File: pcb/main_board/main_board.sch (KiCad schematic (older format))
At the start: 32 parts, among them J1 Sensors_Conn, J2 Power_Conn, J3 I2C_Conn, J4 Garage_Conn, J5 Debug_Sensors_Conn, J6 Debug_I2C_Conn, U1 ESP-01, U2 HC_05, U3 AT24CS64-SSHM, U4 AMS1117-3.3, U5 Black_Pill

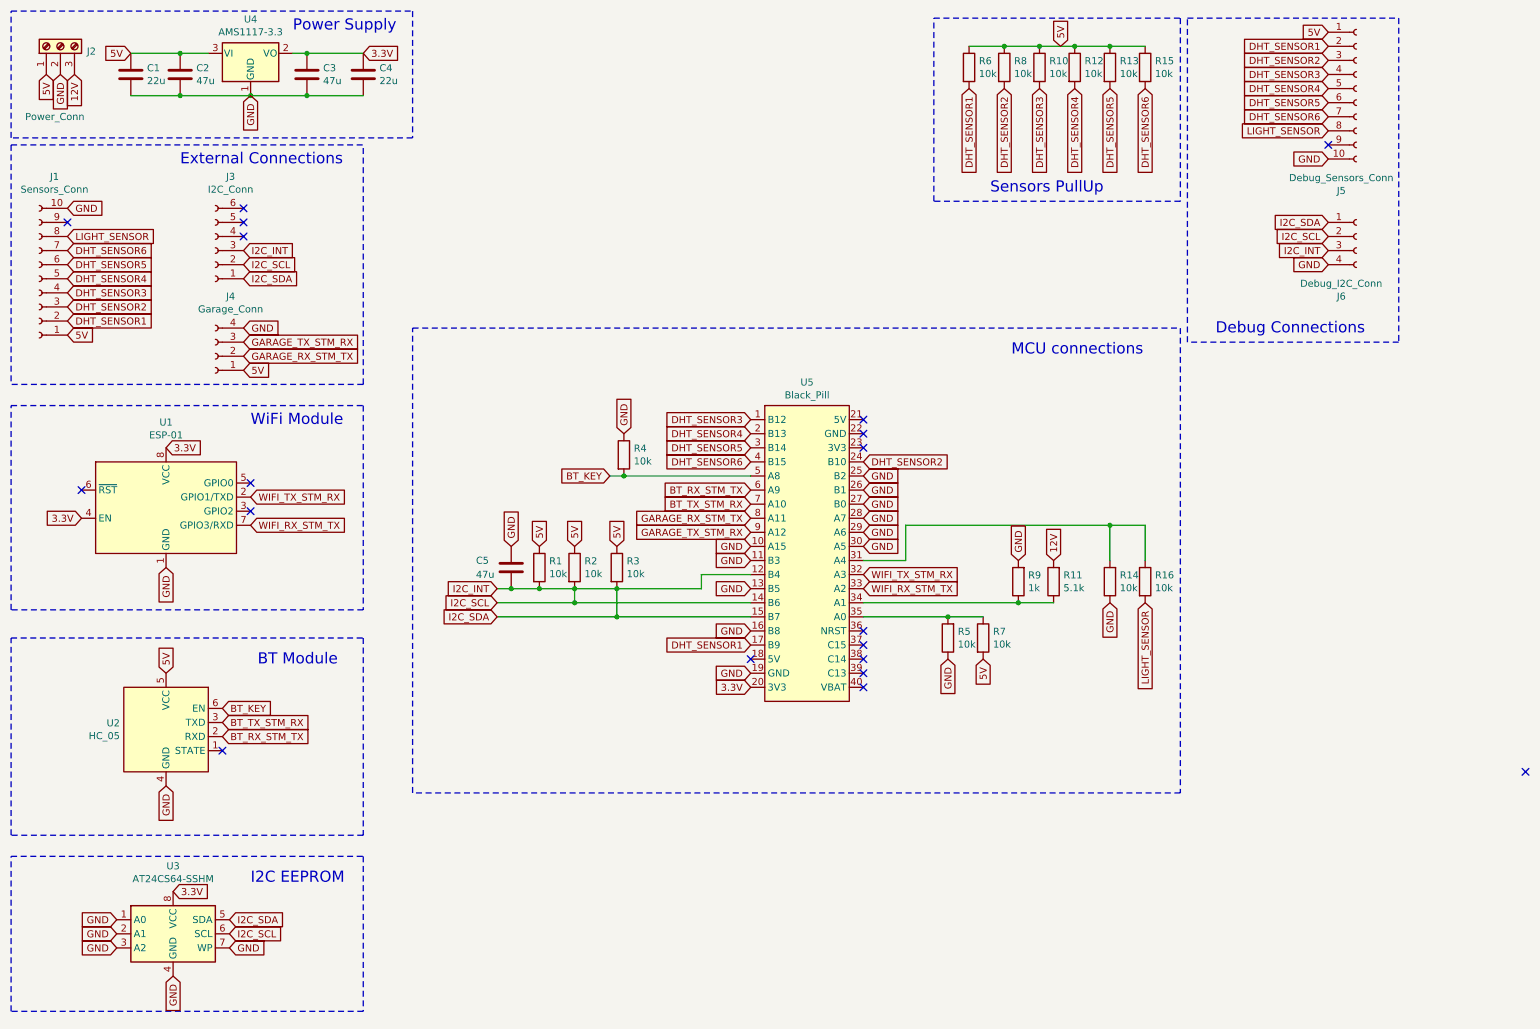
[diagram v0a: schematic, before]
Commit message: PCB layout added
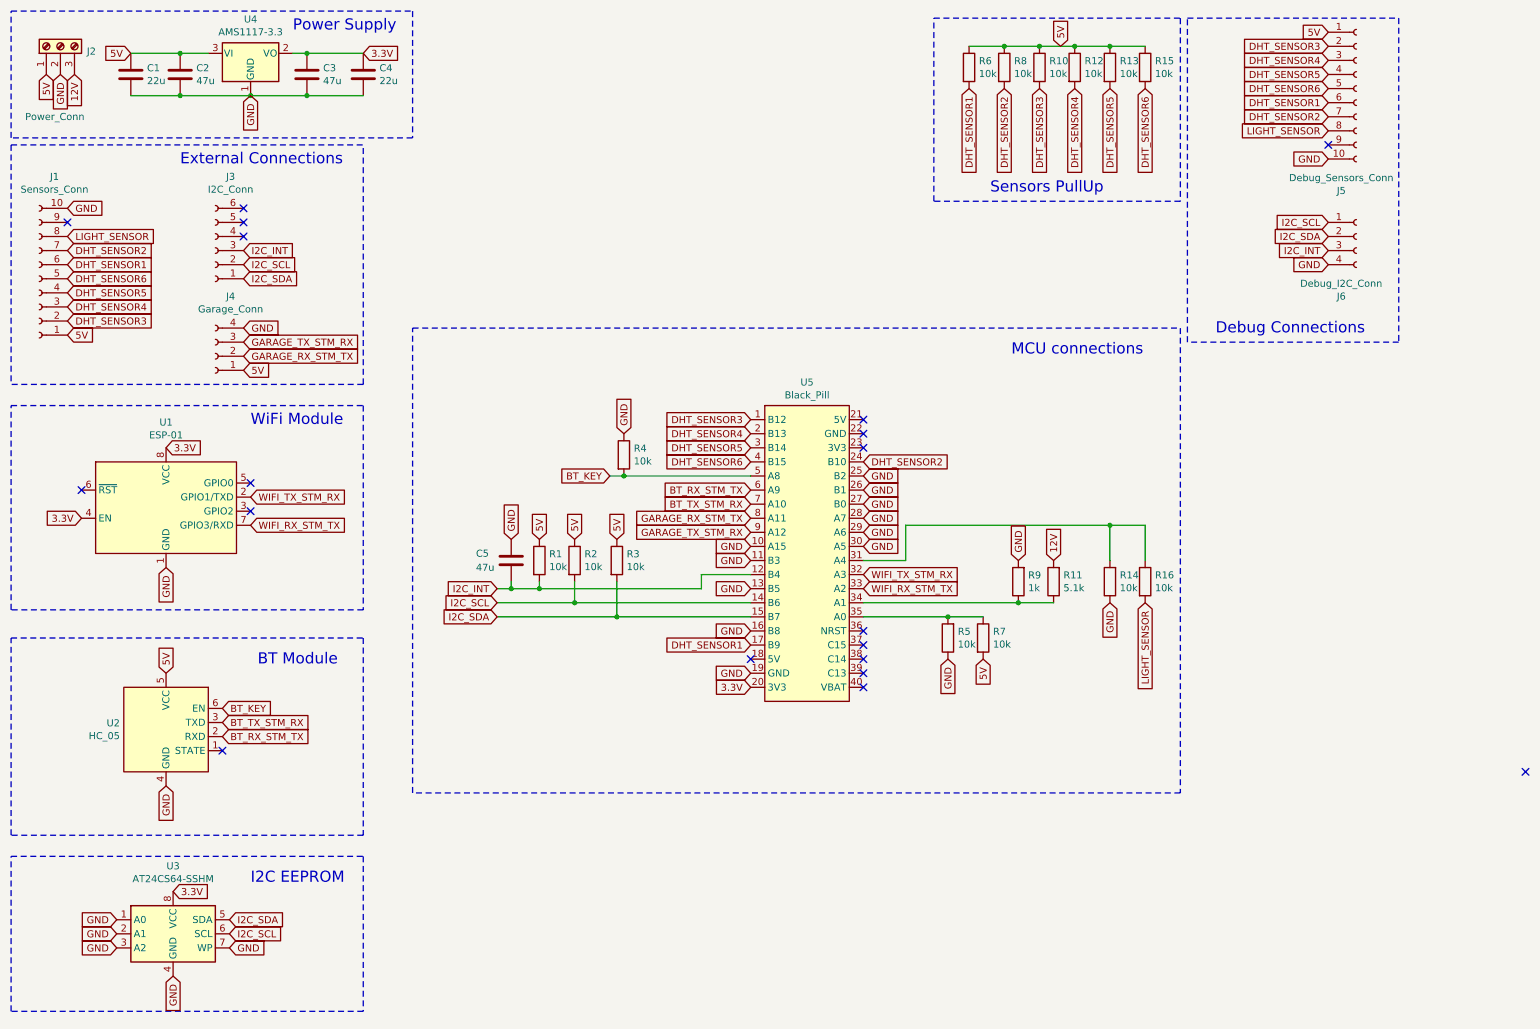
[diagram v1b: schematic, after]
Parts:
- U1: footprint Connector_PinHeader_2.54mm:PinHeader_2x04_P2.54mm_Vertical -> project_footprints:ESP01
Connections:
- net DHT_SENSOR1: now also J1.6 (Pin_6), J5.6 (Pin_6); no longer J1.2 (Pin_2), J5.2 (Pin_2)
- net DHT_SENSOR2: now also J1.7 (Pin_7), J5.7 (Pin_7); no longer J1.3 (Pin_3), J5.3 (Pin_3)
- net DHT_SENSOR3: now also J1.2 (Pin_2), J5.2 (Pin_2); no longer J1.4 (Pin_4), J5.4 (Pin_4)
- net DHT_SENSOR4: now also J1.3 (Pin_3), J5.3 (Pin_3); no longer J1.5 (Pin_5), J5.5 (Pin_5)
- net DHT_SENSOR5: now also J1.4 (Pin_4), J5.4 (Pin_4); no longer J1.6 (Pin_6), J5.6 (Pin_6)
- net DHT_SENSOR6: now also J1.5 (Pin_5), J5.5 (Pin_5); no longer J1.7 (Pin_7), J5.7 (Pin_7)
- net I2C_INT: no longer J3.1 (Pin_1), J3.2 (Pin_2), J6.1 (Pin_1), J6.2 (Pin_2), R2.2, R3.2, U3.5 (SDA), U3.6 (SCL), U5.14 (B6), U5.15 (B7)
- new net I2C_SCL: J3.2 (Pin_2), J6.1 (Pin_1), R2.2, U3.6 (SCL), U5.14 (B6)
- new net I2C_SDA: J3.1 (Pin_1), J6.2 (Pin_2), R3.2, U3.5 (SDA), U5.15 (B7)
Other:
- moved on the sheet: C5, R1, R2, R3
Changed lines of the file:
@@
 Text GLabel 1750 2800 2    50   Input ~ 0
 5V
+Text GLabel 1750 2300 2    50   Input ~ 0
+DHT_SENSOR1
+Text GLabel 1750 2200 2    50   Input ~ 0
+DHT_SENSOR2
 Text GLabel 1750 2700 2    50   Input ~ 0
-DHT_SENSOR1
+DHT_SENSOR3
 Text GLabel 1750 2600 2    50   Input ~ 0
-DHT_SENSOR2
+DHT_SENSOR4
 Text GLabel 1750 2500 2    50   Input ~ 0
-DHT_SENSOR3
+DHT_SENSOR5
 Text GLabel 1750 2400 2    50   Input ~ 0
-DHT_SENSOR4
-Text GLabel 1750 2300 2    50   Input ~ 0
-DHT_SENSOR5
-Text GLabel 1750 2200 2    50   Input ~ 0
 DHT_SENSOR6
 Text GLabel 1750 2100 2    50   Input ~ 0
@@
 NoConn ~ 3000 2000
 NoConn ~ 3000 2100
-Text GLabel 3000 2200 2    50   Input ~ 0
-I2C_INT
-Text GLabel 3000 2300 2    50   Input ~ 0
-I2C_SCL
 $Comp
 L Connector:Conn_01x04_Female J4
@@
 Text GLabel 3000 2950 2    50   Input ~ 0
 GARAGE_RX_STM_TX
-$Comp
-L project_symbols:ESP-01 U1
-U 1 1 5FFDA57F
-P 2450 4000
-F 0 "U1" H 2450 4581 50  0000 C CNN
-F 1 "ESP-01" H 2450 4490 50  0000 C CNN
-F 2 "Connector_PinHeader_2.54mm:PinHeader_2x04_P2.54mm_Vertical" H 2450 4489 50  0001 C CNN
-F 3 "" H 2100 4100 50  0001 C CNN
-	1    2450 4000
-	1    0    0    -1
-$EndComp
 Text GLabel 2450 4450 3    50   Input ~ 0
 GND
@@
 Text GLabel 2500 6750 2    50   Input ~ 0
 3.3V
-Text GLabel 2900 7050 2    50   Input ~ 0
-I2C_SCL
-Text GLabel 2900 6950 2    50   Input ~ 0
-I2C_SDA
 Wire Notes Line
 	1350 6500 3850 6500
@@
 L Device:R R1
 U 1 1 6004496A
-P 5100 4450
-F 0 "R1" H 5170 4496 50  0000 L CNN
-F 1 "10k" H 5170 4405 50  0000 L CNN
-F 2 "Resistor_SMD:R_1206_3216Metric_Pad1.30x1.75mm_HandSolder" V 5030 4450 50  0001 C CNN
-F 3 "~" H 5100 4450 50  0001 C CNN
-	1    5100 4450
-	1    0    0    -1
-$EndComp
-Text GLabel 5100 4300 1    50   Input ~ 0
-5V
-Text GLabel 4800 4700 0    50   Input ~ 0
-I2C_SCL
+P 5100 4400
+F 0 "R1" H 5170 4446 50  0000 L CNN
+F 1 "10k" H 5170 4355 50  0000 L CNN
+F 2 "Resistor_SMD:R_1206_3216Metric_Pad1.30x1.75mm_HandSolder" V 5030 4400 50  0001 C CNN
+F 3 "~" H 5100 4400 50  0001 C CNN
+	1    5100 4400
+	1    0    0    -1
+$EndComp
+Text GLabel 5100 4250 1    50   Input ~ 0
+5V
 $Comp
 L Connector:Conn_01x06_Female J3
@@
 	-1   0    0    1
 $EndComp
-Text GLabel 3000 2400 2    50   Input ~ 0
-I2C_SDA
-Text GLabel 4800 4800 0    50   Input ~ 0
-I2C_SDA
 $Comp
 L Device:R R3
 U 1 1 6004C3D0
-P 5650 4450
-F 0 "R3" H 5720 4496 50  0000 L CNN
-F 1 "10k" H 5720 4405 50  0000 L CNN
-F 2 "Resistor_SMD:R_1206_3216Metric_Pad1.30x1.75mm_HandSolder" V 5580 4450 50  0001 C CNN
-F 3 "~" H 5650 4450 50  0001 C CNN
-	1    5650 4450
-	1    0    0    -1
-$EndComp
-Text GLabel 5350 4300 1    50   Input ~ 0
-5V
-Text GLabel 5650 4300 1    50   Input ~ 0
-5V
-Text GLabel 4800 4600 0    50   Input ~ 0
-I2C_INT
-Wire Wire Line
-	5350 4600 5350 4700
-Wire Wire Line
-	5650 4600 5650 4800
+P 5650 4400
+F 0 "R3" H 5720 4446 50  0000 L CNN
+F 1 "10k" H 5720 4355 50  0000 L CNN
+F 2 "Resistor_SMD:R_1206_3216Metric_Pad1.30x1.75mm_HandSolder" V 5580 4400 50  0001 C CNN
+F 3 "~" H 5650 4400 50  0001 C CNN
+	1    5650 4400
+	1    0    0    -1
+$EndComp
+Text GLabel 5350 4250 1    50   Input ~ 0
+5V
+Text GLabel 5650 4250 1    50   Input ~ 0
+5V
 $Comp
 L Device:R R5
@@
 Text GLabel 9150 4700 3    50   Input ~ 0
 GND
-Wire Wire Line
-	7400 4400 7700 4400
 Text GLabel 6600 4200 0    50   Input ~ 0
 GARAGE_TX_STM_RX
@@
 Wire Wire Line
 	4800 4600 4900 4600
-Connection ~ 5100 4600
 Wire Wire Line
 	4800 4700 5350 4700
@@
 L Device:C C5
 U 1 1 600B5AF0
-P 4900 4450
-F 0 "C5" H 4650 4500 50  0000 L CNN
-F 1 "47u" H 4650 4400 50  0000 L CNN
-F 2 "Capacitor_THT:CP_Radial_D8.0mm_P2.50mm" H 4938 4300 50  0001 C CNN
-F 3 "~" H 4900 4450 50  0001 C CNN
-	1    4900 4450
+P 4900 4400
+F 0 "C5" H 4650 4450 50  0000 L CNN
+F 1 "47u" H 4650 4350 50  0000 L CNN
+F 2 "Capacitor_THT:CP_Radial_D8.0mm_P2.50mm" H 4938 4250 50  0001 C CNN
+F 3 "~" H 4900 4400 50  0001 C CNN
+	1    4900 4400
 	1    0    0    -1
 $EndComp
 Connection ~ 4900 4600
-Wire Wire Line
-	4900 4600 5100 4600
-Text GLabel 4900 4300 1    50   Input ~ 0
-GND
-Wire Wire Line
-	5100 4600 5350 4600
+Text GLabel 4900 4250 1    50   Input ~ 0
+GND
 $Comp
 L Device:R R2
 U 1 1 6004B406
-P 5350 4450
-F 0 "R2" H 5420 4496 50  0000 L CNN
-F 1 "10k" H 5420 4405 50  0000 L CNN
-F 2 "Resistor_SMD:R_1206_3216Metric_Pad1.30x1.75mm_HandSolder" V 5280 4450 50  0001 C CNN
-F 3 "~" H 5350 4450 50  0001 C CNN
-	1    5350 4450
+P 5350 4400
+F 0 "R2" H 5420 4446 50  0000 L CNN
+F 1 "10k" H 5420 4355 50  0000 L CNN
+F 2 "Resistor_SMD:R_1206_3216Metric_Pad1.30x1.75mm_HandSolder" V 5280 4400 50  0001 C CNN
+F 3 "~" H 5350 4400 50  0001 C CNN
+	1    5350 4400
 	1    0    0    -1
 $EndComp
@@
 Text GLabel 10700 650  0    50   Input ~ 0
 5V
+Text GLabel 10700 1150 0    50   Input ~ 0
+DHT_SENSOR1
+Text GLabel 10700 1250 0    50   Input ~ 0
+DHT_SENSOR2
 Text GLabel 10700 750  0    50   Input ~ 0
-DHT_SENSOR1
+DHT_SENSOR3
 Text GLabel 10700 850  0    50   Input ~ 0
-DHT_SENSOR2
+DHT_SENSOR4
 Text GLabel 10700 950  0    50   Input ~ 0
-DHT_SENSOR3
+DHT_SENSOR5
 Text GLabel 10700 1050 0    50   Input ~ 0
-DHT_SENSOR4
-Text GLabel 10700 1150 0    50   Input ~ 0
-DHT_SENSOR5
-Text GLabel 10700 1250 0    50   Input ~ 0
 DHT_SENSOR6
 Text GLabel 10700 1350 0    50   Input ~ 0
@@
 	1    0    0    -1
 $EndComp
-Text GLabel 10700 2200 0    50   Input ~ 0
-I2C_INT
-Text GLabel 10700 2100 0    50   Input ~ 0
-I2C_SCL
-Text GLabel 10700 2000 0    50   Input ~ 0
-I2C_SDA
 Text GLabel 10700 2300 0    50   Input ~ 0
 GND
@@
 Text Notes 8300 1800 0    79   ~ 0
 Sensors PullUp
-Connection ~ 5350 4600
-Wire Wire Line
-	5350 4600 5650 4600
-Connection ~ 5650 4600
-Wire Wire Line
-	5650 4600 6250 4600
 Wire Notes Line
 	4200 2750 9650 2750
@@
 NoConn ~ 7400 5200
 NoConn ~ 12100 5900
+Text GLabel 10700 2200 0    50   Input ~ 0
+I2C_INT
+Text GLabel 10700 2000 0    50   Input ~ 0
+I2C_SCL
+Text GLabel 10700 2100 0    50   Input ~ 0
+I2C_SDA
+Text GLabel 2900 6950 2    50   Input ~ 0
+I2C_SDA
+Text GLabel 2900 7050 2    50   Input ~ 0
+I2C_SCL
+Text GLabel 4800 4800 0    50   Input ~ 0
+I2C_SDA
+Text GLabel 4800 4700 0    50   Input ~ 0
+I2C_SCL
+Text GLabel 4800 4600 0    50   Input ~ 0
+I2C_INT
+Text GLabel 3000 2200 2    50   Input ~ 0
+I2C_INT
+Text GLabel 3000 2400 2    50   Input ~ 0
+I2C_SDA
+Text GLabel 3000 2300 2    50   Input ~ 0
+I2C_SCL
+Wire Wire Line
+	4900 4600 5100 4600
+Wire Wire Line
+	4900 4550 4900 4600
+Wire Wire Line
+	5100 4550 5100 4600
+Connection ~ 5100 4600
+Wire Wire Line
+	5650 4550 5650 4800
+Wire Wire Line
+	5350 4550 5350 4700
+Wire Wire Line
+	5100 4600 6250 4600
+$Comp
+L project_symbols:ESP-01 U1
+U 1 1 5FFDA57F
+P 2450 4000
+F 0 "U1" H 2450 4581 50  0000 C CNN
+F 1 "ESP-01" H 2450 4490 50  0000 C CNN
+F 2 "project_footprints:ESP01" H 2450 4489 50  0001 C CNN
+F 3 "" H 2100 4100 50  0001 C CNN
+	1    2450 4000
+	1    0    0    -1
+$EndComp
+Wire Wire Line
+	7400 4400 7700 4400
 $EndSCHEMATC
